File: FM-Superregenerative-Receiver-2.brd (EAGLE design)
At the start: 25.4 x 30.5 mm, 17 parts, among them T1 BC547

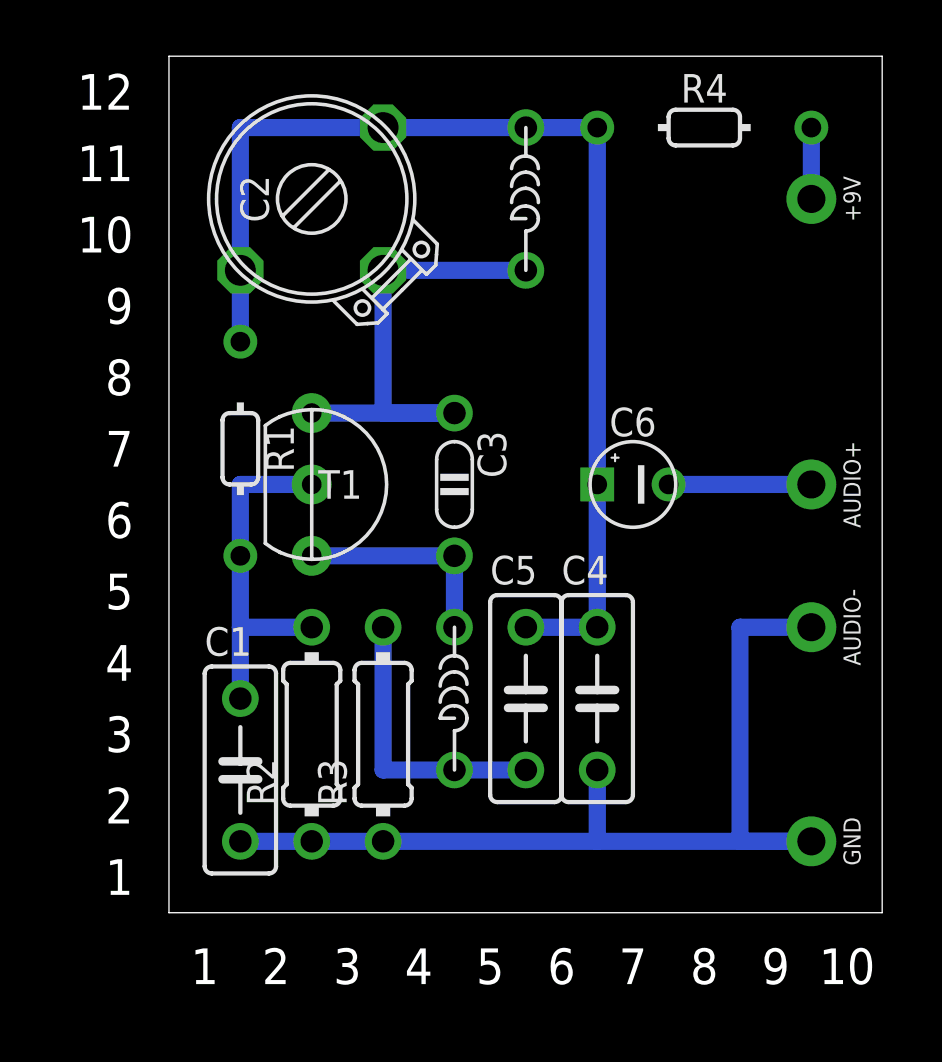
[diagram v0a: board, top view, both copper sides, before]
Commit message: ...
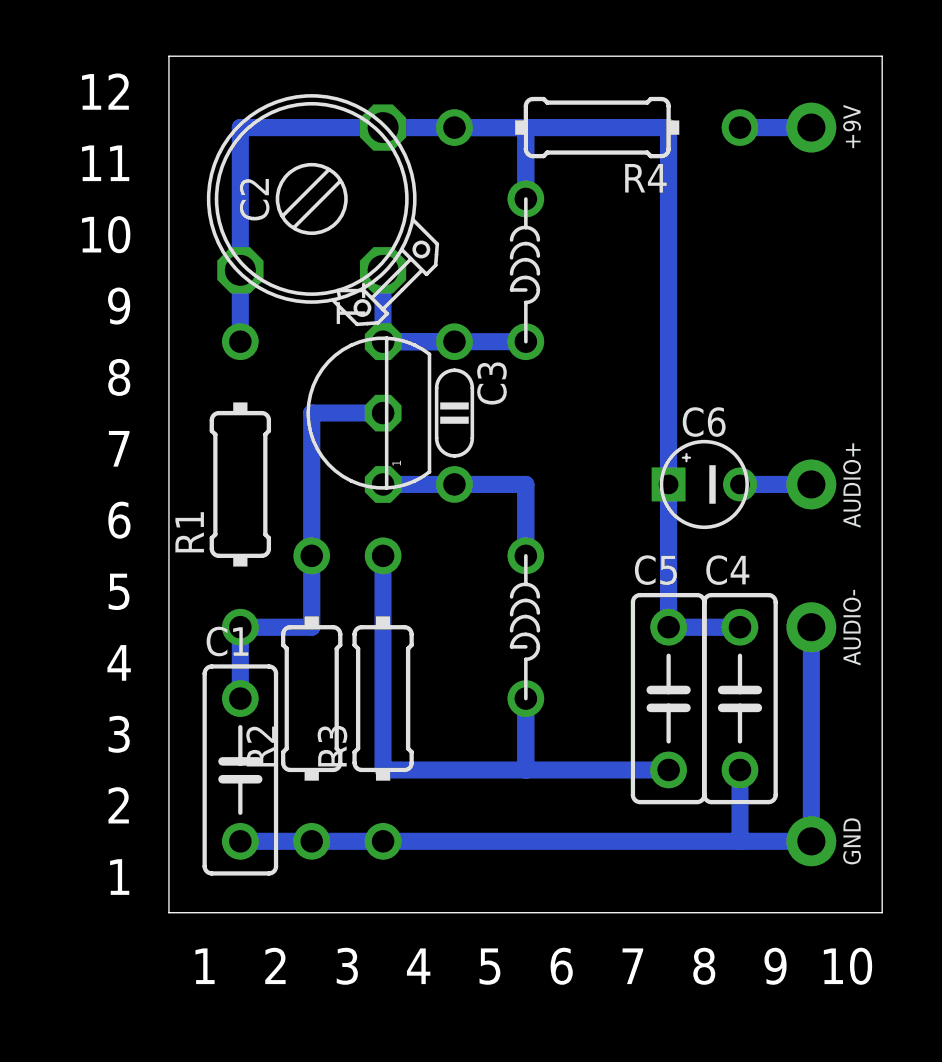
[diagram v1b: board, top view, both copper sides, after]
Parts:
- R1, R4: device r:0202/7 -> r:0204/10
- R2, R3: device r:0204/7 -> r:0204/10
- T1: value BC547 -> 2N3904; device t:TO92-CBE -> t:TO92
- moved C5 5.08 mm to (17.8, 7.62)
- moved C4 5.08 mm to (20.3, 7.62)
- moved R4 3.81 mm to (15.2, 27.9), turned to 180 degrees
- moved T1 3.59 mm to (7.62, 17.8), turned to 90 degrees
- moved L2 3.59 mm to (12.7, 10.2)
- moved +9V 2.54 mm to (22.9, 27.9)
- moved C3 2.54 mm to (10.2, 17.8)
- moved C6 2.54 mm to (19.1, 15.2)
- moved L1 2.54 mm to (12.7, 22.9)
- moved R1 1.27 mm to (2.54, 15.2), turned to 90 degrees
- moved R2 1.27 mm to (5.08, 7.62)
- moved R3 1.27 mm to (7.62, 7.62)
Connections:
- net N$1: now also T1.2; no longer T1.B
- net N$4: now also T1.1; no longer T1.E
- net N$6: now also T1.3; no longer T1.C
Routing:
- net N$3: track 10.2 -> 20.3 mm
- net N$8: track 40.6 -> 48.3 mm
- net N$6: track 17.8 -> 10.2 mm
- net GND: track 35.6 -> 30.5 mm
- net N$1: track 12.7 -> 15.2 mm
- net N$2: track 5.08 -> 2.54 mm
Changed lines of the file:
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@@
 </autorouter>
 <elements>
-<element name="+9V" library="pad" package="SPAD" value="SPAD" x="22.86" y="25.4" rot="R180"/>
+<element name="+9V" library="pad" package="SPAD" value="SPAD" x="22.86" y="27.94" rot="R180"/>
 <element name="AUDIO+" library="pad" package="SPAD" value="SPAD" x="22.86" y="15.24" rot="R180"/>
 <element name="C1" library="c" package="C050-025X075" value="10n" x="2.54" y="5.08" rot="R90"/>
 <element name="C2" library="cap-trim" package="TRIM-2222-808" value="22p" x="5.08" y="25.4" rot="R90"/>
-<element name="C3" library="c" package="C050-020X036" value="10p" x="10.16" y="15.24" rot="R270"/>
-<element name="C4" library="c" package="C050-025X075" value="10n" x="15.24" y="7.62" rot="R90"/>
-<element name="C5" library="c" package="C050-025X075" value="10n" x="12.7" y="7.62" rot="R90"/>
-<element name="C6" library="c" package="E2,5-3" value="10u" x="16.51" y="15.24" rot="R90"/>
-<element name="L1" library="r" package="L-02/5V" value="5" x="12.7" y="25.4"/>
-<element name="L2" library="r" package="L-02/5V" value="0.33uH" x="10.16" y="7.62"/>
-<element name="R1" library="r" package="0202/7" value="10k" x="2.54" y="16.51" rot="R180"/>
-<element name="R2" library="r" package="0204/7" value="10k" x="5.08" y="6.35" rot="R90"/>
-<element name="R3" library="r" package="0204/7" value="10k" x="7.62" y="6.35" rot="R90"/>
-<element name="R4" library="r" package="0202/7" value="10k" x="19.05" y="27.94" rot="R270"/>
-<element name="T1" library="t" package="TO92-CBE" value="BC547" x="5.08" y="15.24"/>
+<element name="C3" library="c" package="C050-020X036" value="10p" x="10.16" y="17.78" rot="R270"/>
+<element name="C4" library="c" package="C050-025X075" value="10n" x="20.32" y="7.62" rot="R90"/>
+<element name="C5" library="c" package="C050-025X075" value="10n" x="17.78" y="7.62" rot="R90"/>
+<element name="C6" library="c" package="E2,5-3" value="10u" x="19.05" y="15.24" rot="R90"/>
+<element name="L1" library="r" package="L-02/5V" value="5" x="12.7" y="22.86"/>
+<element name="L2" library="r" package="L-02/5V" value="0.33uH" x="12.7" y="10.16"/>
+<element name="R1" library="r" package="0204/10" value="10k" x="2.54" y="15.24" rot="R90"/>
+<element name="R2" library="r" package="0204/10" value="10k" x="5.08" y="7.62" rot="R90"/>
+<element name="R3" library="r" package="0204/10" value="10k" x="7.62" y="7.62" rot="R90"/>
+<element name="R4" library="r" package="0204/10" value="10k" x="15.24" y="27.94" rot="R180"/>
+<element name="T1" library="t" package="TO92" value="2N3904" x="7.62" y="17.78" rot="R90"/>
 <element name="GND" library="pad" package="SPAD" value="SPAD" x="22.86" y="2.54" rot="R180"/>
 <element name="AUDIO-" library="pad" package="SPAD" value="SPAD" x="22.86" y="10.16" rot="R180"/>
@@
 <contactref element="R2" pad="2"/>
 <contactref element="R1" pad="1"/>
-<contactref element="T1" pad="B"/>
-<wire x1="2.54" y1="12.7" x2="2.54" y2="15.24" width="0.6096" layer="16"/>
-<wire x1="2.54" y1="15.24" x2="5.08" y2="15.24" width="0.6096" layer="16"/>
-<wire x1="2.54" y1="12.7" x2="2.54" y2="10.16" width="0.6096" layer="16"/>
+<contactref element="T1" pad="2"/>
+<wire x1="5.08" y1="12.7" x2="5.08" y2="17.78" width="0.6096" layer="16"/>
+<wire x1="5.08" y1="17.78" x2="7.62" y2="17.78" width="0.6096" layer="16"/>
 <wire x1="2.54" y1="7.62" x2="2.54" y2="10.16" width="0.6096" layer="16"/>
 <wire x1="2.54" y1="10.16" x2="5.08" y2="10.16" width="0.6096" layer="16"/>
+<wire x1="5.08" y1="10.16" x2="5.08" y2="12.7" width="0.6096" layer="16"/>
+<wire x1="2.54" y1="7.62" x2="2.54" y2="10.16" width="0" layer="19" extent="1-1"/>
 </signal>
 <signal name="N$3">
@@
 <contactref element="R3" pad="2"/>
 <contactref element="C5" pad="2"/>
-<wire x1="12.7" y1="5.08" x2="10.16" y2="5.08" width="0.6096" layer="16"/>
-<wire x1="10.16" y1="5.08" x2="7.62" y2="5.08" width="0.6096" layer="16"/>
-<wire x1="7.62" y1="5.08" x2="7.62" y2="10.16" width="0.6096" layer="16"/>
+<wire x1="17.78" y1="5.08" x2="12.7" y2="5.08" width="0.6096" layer="16"/>
+<wire x1="12.7" y1="7.62" x2="12.7" y2="5.08" width="0.6096" layer="16"/>
+<wire x1="12.7" y1="5.08" x2="7.62" y2="5.08" width="0.6096" layer="16"/>
+<wire x1="7.62" y1="5.08" x2="7.62" y2="12.7" width="0.6096" layer="16"/>
 </signal>
 <signal name="N$4">
-<contactref element="T1" pad="E"/>
+<contactref element="T1" pad="1"/>
 <contactref element="L2" pad="1"/>
 <contactref element="C3" pad="2"/>
-<wire x1="10.16" y1="12.7" x2="5.08" y2="12.7" width="0.6096" layer="16"/>
-<wire x1="10.16" y1="10.16" x2="10.16" y2="12.7" width="0.6096" layer="16"/>
+<wire x1="10.16" y1="15.24" x2="7.62" y2="15.24" width="0.6096" layer="16"/>
+<wire x1="12.7" y1="12.7" x2="12.7" y2="15.24" width="0.6096" layer="16"/>
+<wire x1="12.7" y1="15.24" x2="10.16" y2="15.24" width="0.6096" layer="16"/>
 </signal>
 <signal name="N$6">
 <contactref element="C2" pad="2"/>
 <contactref element="L1" pad="2"/>
-<contactref element="T1" pad="C"/>
+<contactref element="T1" pad="3"/>
 <contactref element="C3" pad="1"/>
-<wire x1="10.16" y1="17.78" x2="5.08" y2="17.78" width="0.6096" layer="16"/>
-<wire x1="7.62" y1="22.86" x2="7.62" y2="17.78" width="0.6096" layer="16"/>
-<wire x1="7.62" y1="17.78" x2="10.16" y2="17.78" width="0.6096" layer="16"/>
-<wire x1="12.7" y1="22.86" x2="7.62" y2="22.86" width="0.6096" layer="16"/>
+<wire x1="7.62" y1="20.32" x2="10.16" y2="20.32" width="0.6096" layer="16"/>
+<wire x1="12.7" y1="20.32" x2="7.62" y2="20.32" width="0.6096" layer="16"/>
+<wire x1="7.62" y1="20.32" x2="7.62" y2="22.86" width="0.6096" layer="16"/>
 </signal>
 <signal name="N$8">
@@
 <wire x1="2.54" y1="27.94" x2="2.54" y2="22.86" width="0.6096" layer="16"/>
 <wire x1="2.54" y1="22.86" x2="2.54" y2="20.32" width="0.6096" layer="16"/>
-<wire x1="12.7" y1="10.16" x2="15.24" y2="10.16" width="0.6096" layer="16"/>
-<wire x1="15.24" y1="10.16" x2="15.24" y2="15.24" width="0.6096" layer="16"/>
-<wire x1="15.24" y1="27.94" x2="12.7" y2="27.94" width="0.6096" layer="16"/>
-<wire x1="12.7" y1="27.94" x2="7.62" y2="27.94" width="0.6096" layer="16"/>
-<wire x1="15.24" y1="15.24" x2="15.24" y2="27.94" width="0.6096" layer="16"/>
+<wire x1="20.32" y1="10.16" x2="17.78" y2="10.16" width="0.6096" layer="16"/>
+<wire x1="17.78" y1="10.16" x2="17.78" y2="15.24" width="0.6096" layer="16"/>
+<wire x1="12.7" y1="25.4" x2="12.7" y2="27.94" width="0.6096" layer="16"/>
+<wire x1="12.7" y1="27.94" x2="10.16" y2="27.94" width="0.6096" layer="16"/>
+<wire x1="10.16" y1="27.94" x2="7.62" y2="27.94" width="0.6096" layer="16"/>
+<wire x1="17.78" y1="15.24" x2="17.78" y2="27.94" width="0.6096" layer="16"/>
+<wire x1="17.78" y1="27.94" x2="10.16" y2="27.94" width="0.6096" layer="16"/>
 </signal>
 <signal name="GND">
@@
 <contactref element="C4" pad="2"/>
 <wire x1="2.54" y1="2.54" x2="5.08" y2="2.54" width="0.6096" layer="16"/>
-<wire x1="7.62" y1="2.54" x2="15.24" y2="2.54" width="0.6096" layer="16"/>
-<wire x1="15.24" y1="2.54" x2="15.24" y2="5.08" width="0.6096" layer="16"/>
+<wire x1="7.62" y1="2.54" x2="20.32" y2="2.54" width="0.6096" layer="16"/>
+<wire x1="20.32" y1="2.54" x2="20.32" y2="5.08" width="0.6096" layer="16"/>
 <contactref element="GND" pad="1"/>
 <contactref element="AUDIO-" pad="1"/>
-<wire x1="22.86" y1="2.54" x2="15.24" y2="2.54" width="0.6096" layer="16"/>
+<wire x1="22.86" y1="2.54" x2="20.32" y2="2.54" width="0.6096" layer="16"/>
 <wire x1="5.08" y1="2.54" x2="7.62" y2="2.54" width="0.6096" layer="16"/>
-<wire x1="22.86" y1="2.54" x2="20.32" y2="2.54" width="0.6096" layer="16"/>
-<wire x1="20.32" y1="2.54" x2="20.32" y2="10.16" width="0.6096" layer="16"/>
-<wire x1="20.32" y1="10.16" x2="22.86" y2="10.16" width="0.6096" layer="16"/>
+<wire x1="22.86" y1="2.54" x2="22.86" y2="10.16" width="0.6096" layer="16"/>
 </signal>
 <signal name="N$7">
 <contactref element="+9V" pad="1"/>
 <contactref element="R4" pad="1"/>
-<wire x1="22.86" y1="25.4" x2="22.86" y2="27.94" width="0.6096" layer="16"/>
+<wire x1="22.86" y1="27.94" x2="20.32" y2="27.94" width="0.6096" layer="16"/>
 </signal>
 <signal name="N$2">
 <contactref element="AUDIO+" pad="1"/>
 <contactref element="C6" pad="-"/>
-<wire x1="17.78" y1="15.24" x2="22.86" y2="15.24" width="0.6096" layer="16"/>
+<wire x1="20.32" y1="15.24" x2="22.86" y2="15.24" width="0.6096" layer="16"/>
 </signal>
 </signals>
